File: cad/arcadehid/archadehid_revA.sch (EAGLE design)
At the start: 30 parts, among them IC1 STM32F10XCXT6, IC3 AMS1117-3.3, X1 8MHz, X2 32.768kHz, X3 USB-MINIB

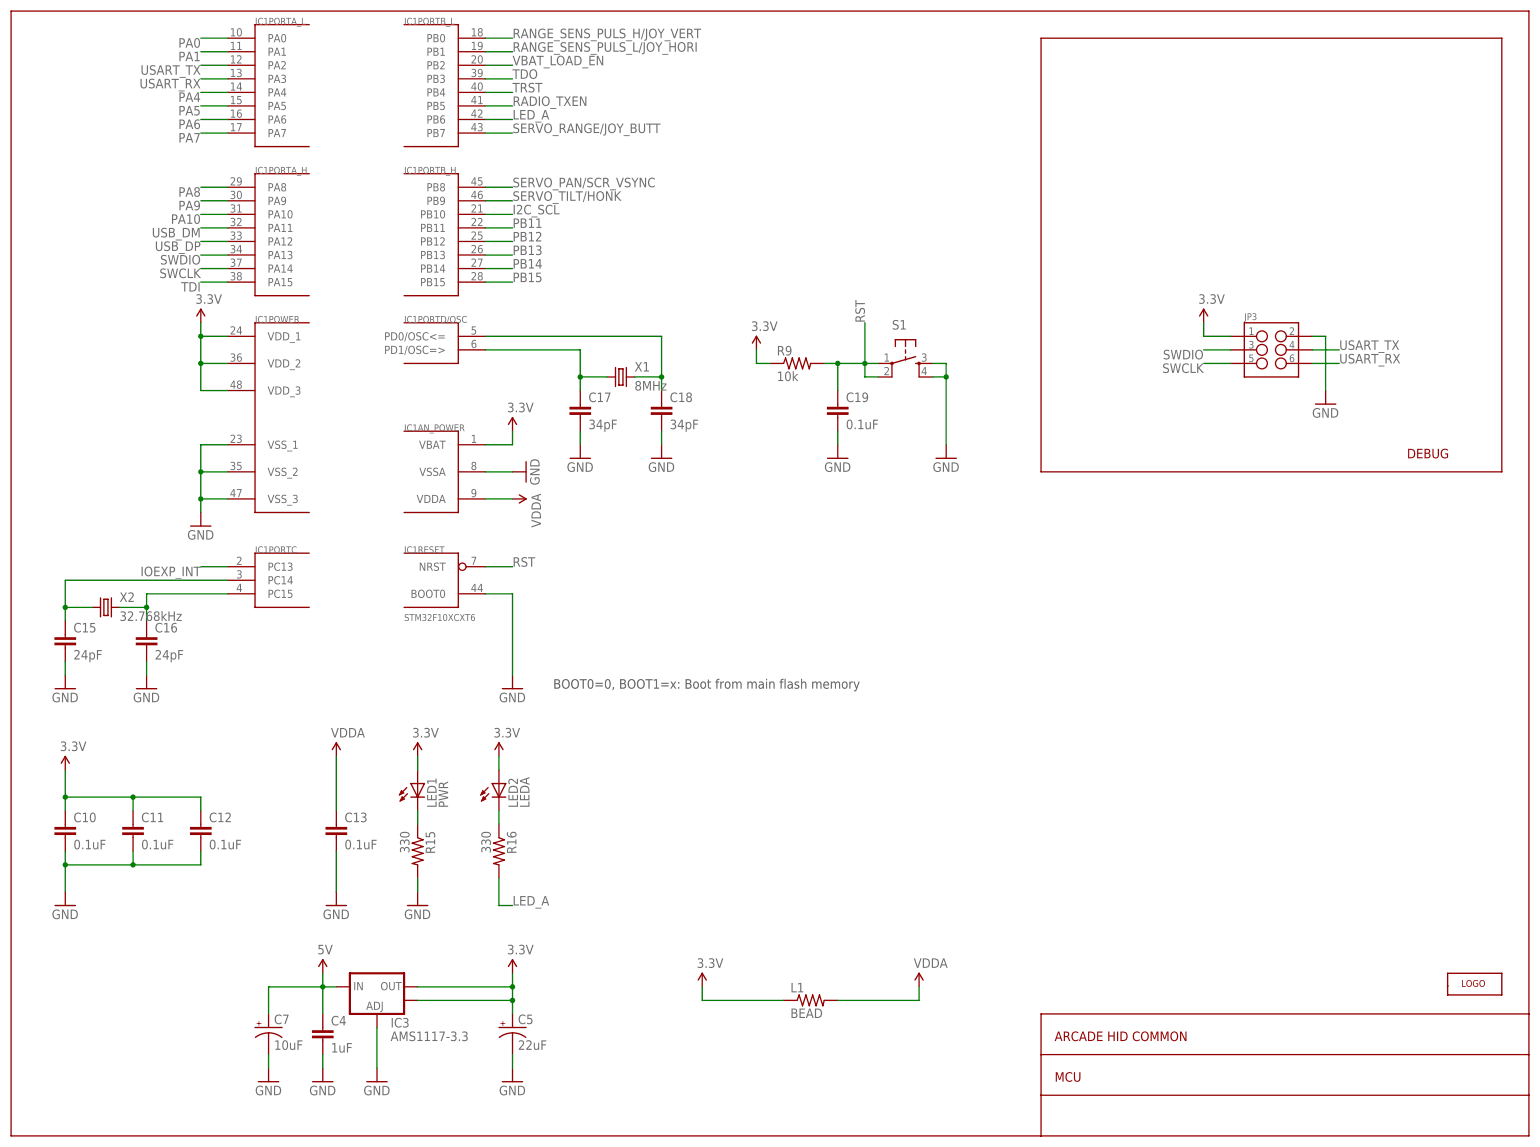
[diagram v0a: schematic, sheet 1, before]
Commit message: cadding, almost there
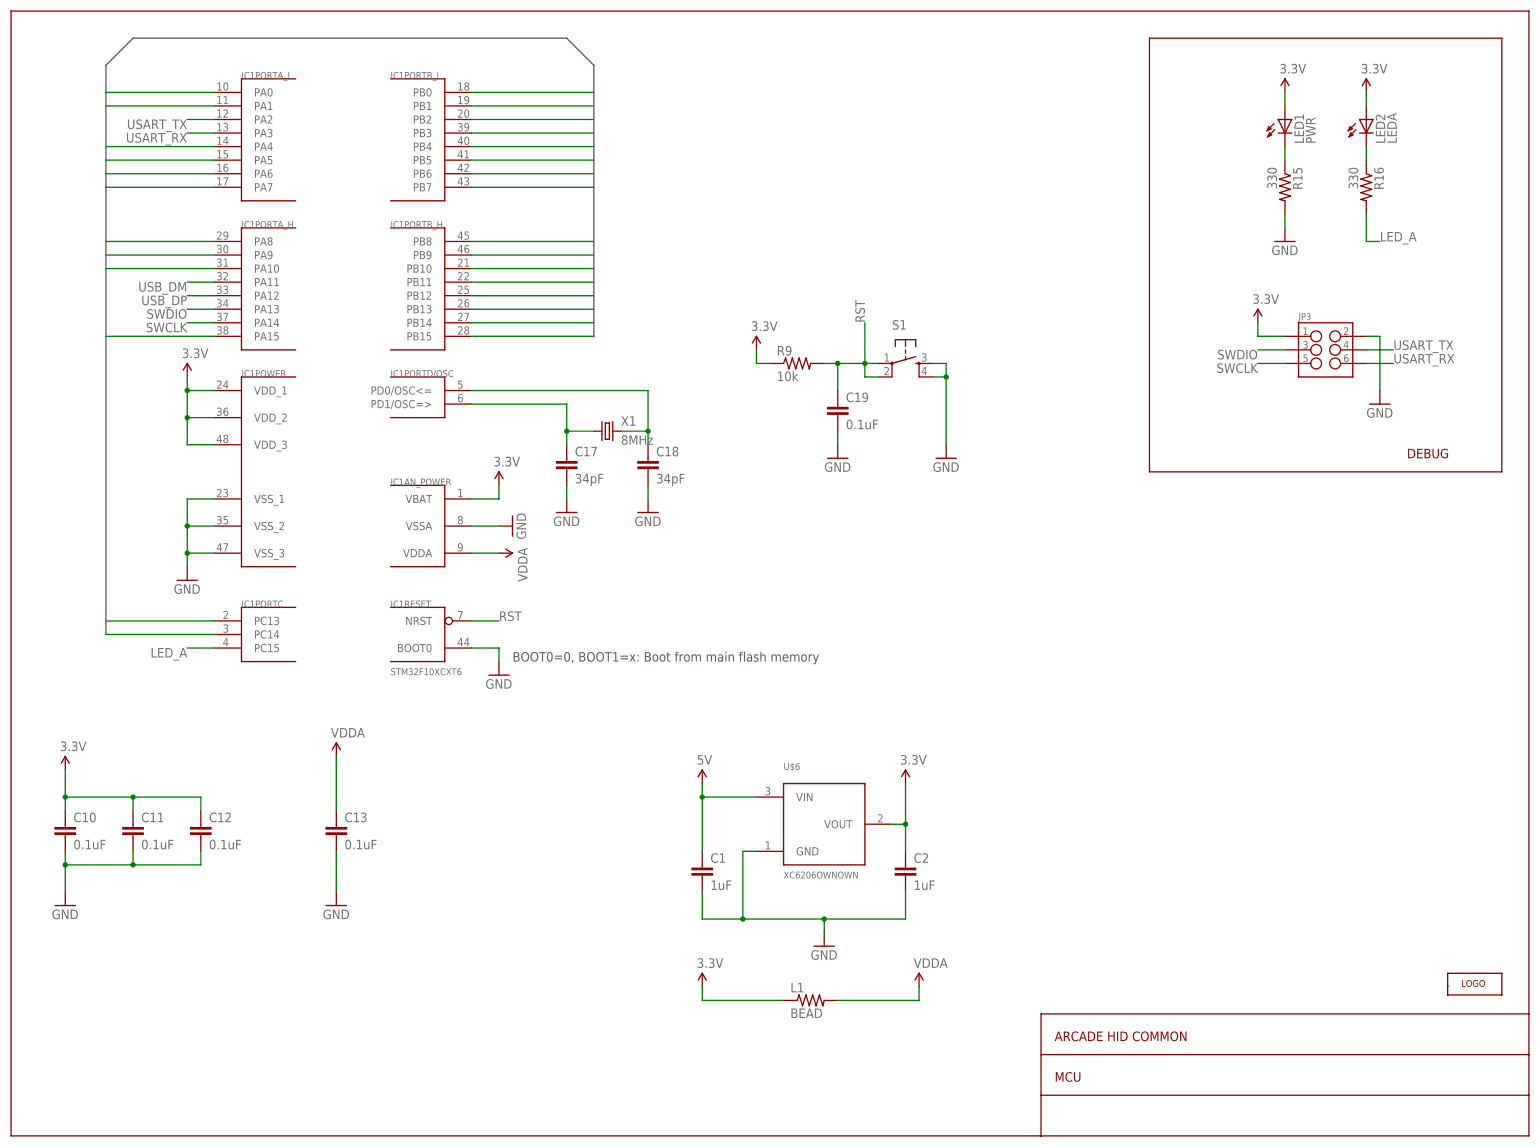
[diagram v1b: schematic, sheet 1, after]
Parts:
- removed C15, C16: 24pF, robot:CAP0402
- removed C4: 1uF, robot:CAP0805
- removed C5: 22uF, robot:CAP_POL1206_CASE-A
- removed C7: 10uF, robot:CAP_POL1206_CASE-A
- removed IC3: AMS1117-3.3, SparkFunEagle-6-6-07:V_REG_LM1117SOT223
- removed U$4, U$5: M08X2, SparkFun-Connectors:M08X2
- removed X2: 32.768kHz, robot:CRYSTALOWN8X4_ACT
- added C1, C2: 1uF, robot:CAP0805
- added C3: 0.1uF, robot:CAP0402
- added JP1, JP2: M13X22X13, SparkFun-Connectors:M13X22X13
- added R10, R11, R12, R13, R14, R17, R18, R19, R20, R21, R22, R23, R24, R25, R26, R27, R28, R29, R3, R30, R31, R4, R5, R6, R7, R8: 30k, SparkFunEagle-6-6-07:RESISTOR0402
- added U$2: MEMORYI2COWN, robot:MEMORYI2COWN
- added U$6: XC6206OWNOWN, robot:XC6206OWNOWN
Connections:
- removed net I2C_SCL: IC1PORTB_H.PB10
- removed net IOEXP_INT: IC1PORTC.PC13
- removed net N$18: U$5.16
- removed net RADIO_TXEN: IC1PORTB_L.PB5
- removed net RANGE_SENS_PULS_H/JOY_VERT: IC1PORTB_L.PB0
- removed net RANGE_SENS_PULS_L/JOY_HORI: IC1PORTB_L.PB1
- removed net RTCI: C15.1, IC1PORTC.PC14, X2.1
- removed net RTCO: C16.1, IC1PORTC.PC15, X2.2
- removed net SERVO_PAN/SCR_VSYNC: IC1PORTB_H.PB8
- removed net SERVO_RANGE/JOY_BUTT: IC1PORTB_L.PB7
- removed net SERVO_TILT/HONK: IC1PORTB_H.PB9
- removed net TDI: IC1PORTA_H.PA15
- removed net TDO: IC1PORTB_L.PB3
- removed net TRST: IC1PORTB_L.PB4
- removed net VBAT_LOAD_EN: IC1PORTB_L.PB2
- new net PA15: IC1PORTA_H.PA15, JP1.16, R11.2
- new net PB0: IC1PORTB_L.PB0, JP2.9, R23.1
- new net PB1: IC1PORTB_L.PB1, JP2.7, R22.1
- new net PB10: IC1PORTB_H.PB10, JP2.3, R20.1
- new net PB2: IC1PORTB_L.PB2, JP2.5, R21.1
- new net PB3: IC1PORTB_L.PB3, JP1.18, R12.2
- new net PB4: IC1PORTB_L.PB4, JP1.20, R13.2
- new net PB5: IC1PORTB_L.PB5, JP1.22, R14.2
- new net PB6: IC1PORTB_L.PB6, JP1.24, R17.2
- new net PB7: IC1PORTB_L.PB7, JP1.26, R18.2
- new net PB8: IC1PORTB_H.PB8, U$2.SCL
- new net PB9: IC1PORTB_H.PB9, U$2.SDA
- new net PC13: IC1PORTC.PC13, JP2.25, R31.1
- new net PC14: IC1PORTC.PC14, JP2.23, R30.1
- net 3.3V: now also C2.1, C3.1, R10.1, R11.1, R12.1, R13.1, R14.1, R17.1, R18.1, R19.2, R20.2, R21.2, R22.2, R23.2, R24.2, R25.2, R26.2, R27.2, R28.2, R29.2, R3.1, R30.2, R31.2, R4.1, R5.1, R6.1, R7.1, R8.1, U$2.VCC, U$6.VOUT; no longer C5.+, IC3.OUT, IC3.OUT@1
- net 5V: now also C1.1, U$6.VIN; no longer C4.1, C7.+, IC3.IN
- net GND: now also C1.2, C2.2, C3.2, JP1.1, JP1.11, JP1.13, JP1.15, JP1.17, JP1.19, JP1.21, JP1.23, JP1.25, JP1.3, JP1.5, JP1.7, JP1.9, JP2.10, JP2.12, JP2.14, JP2.16, JP2.18, JP2.2, JP2.20, JP2.22, JP2.24, JP2.26, JP2.4, JP2.6, JP2.8, U$2./WC, U$2.E1, U$2.E2, U$2.GND, U$6.GND; no longer C15.2, C16.2, C4.2, C5.-, C7.-, IC3.ADJ
- net LED_A: now also IC1PORTC.PC15; no longer IC1PORTB_L.PB6
- net PA0: now also JP2.21, R29.1; no longer U$4.1
- net PA1: now also JP2.19, R28.1; no longer U$4.3
- net PA10: now also JP1.14, R10.2; no longer U$5.6
- net PA4: now also JP2.17, R27.1; no longer U$4.9
- net PA5: now also JP2.15, R26.1; no longer U$4.11
- net PA6: now also JP2.13, R25.1; no longer U$4.13
- net PA7: now also JP2.11, R24.1; no longer U$4.15
- net PA8: now also JP1.10, R7.2; no longer U$5.2
- net PA9: now also JP1.12, R8.2; no longer U$5.4
- net PB11: now also JP2.1, R19.1; no longer U$5.8
- net PB12: now also JP1.2, R3.2; no longer U$5.10
- net PB13: now also JP1.4, R4.2; no longer U$5.12
- net PB14: now also JP1.6, R5.2; no longer U$5.14
- net PB15: now also JP1.8, R6.2
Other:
- moved on the sheet: C17, C18, IC1AN_POWER, IC1PORTA_H, IC1PORTA_L, IC1PORTB_H, IC1PORTB_L, IC1PORTC, IC1PORTD/OSC, IC1POWER, IC1RESET, JP3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
